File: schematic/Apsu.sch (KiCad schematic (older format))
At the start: 34 parts

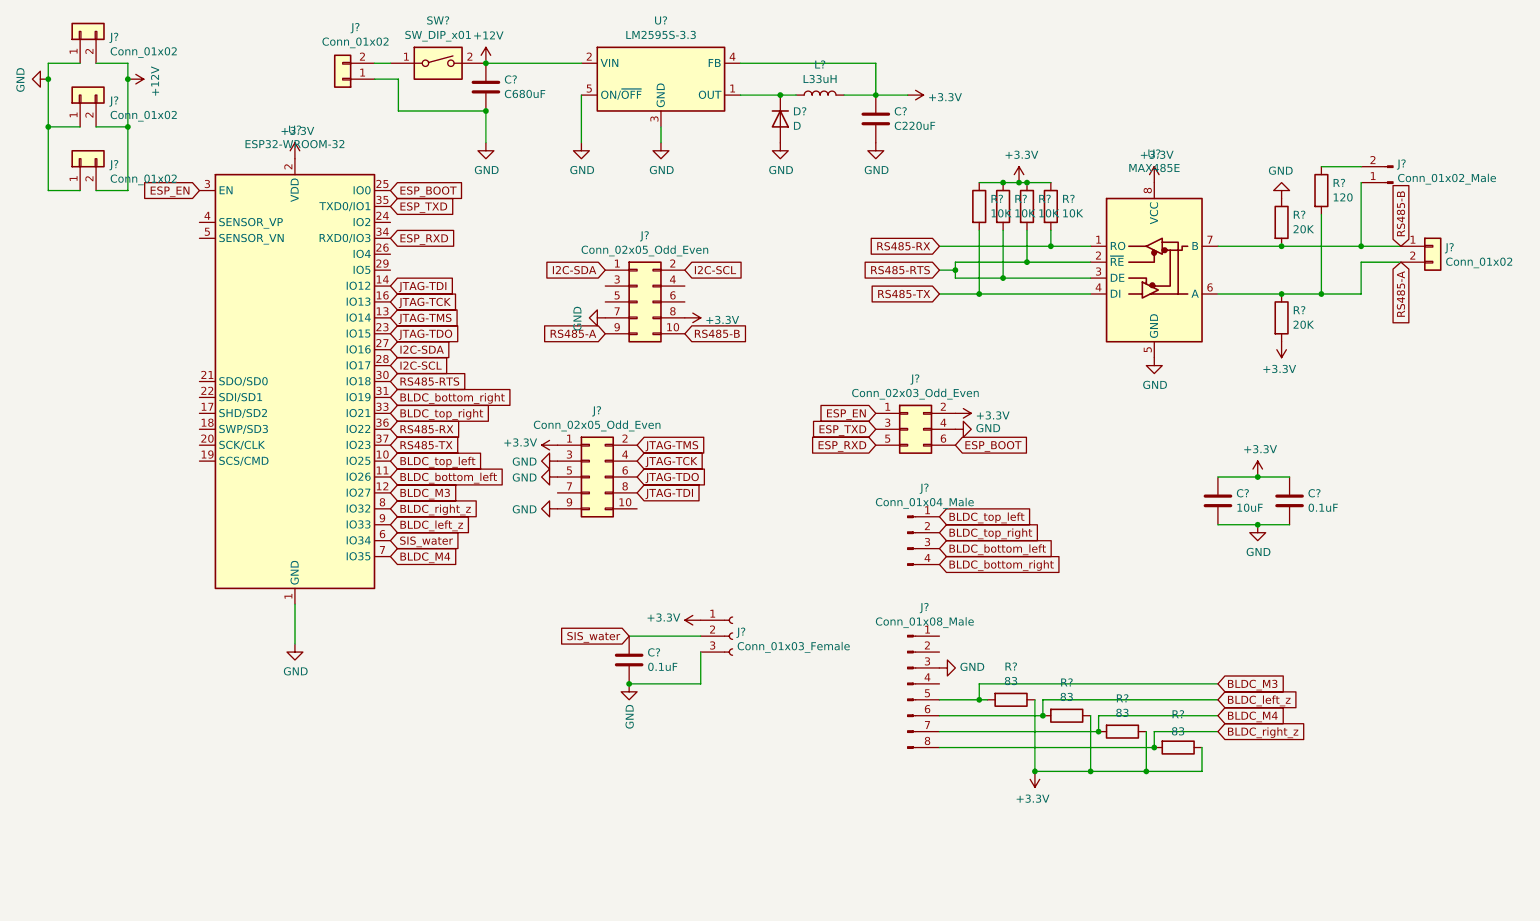
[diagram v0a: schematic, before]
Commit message: dingentjes
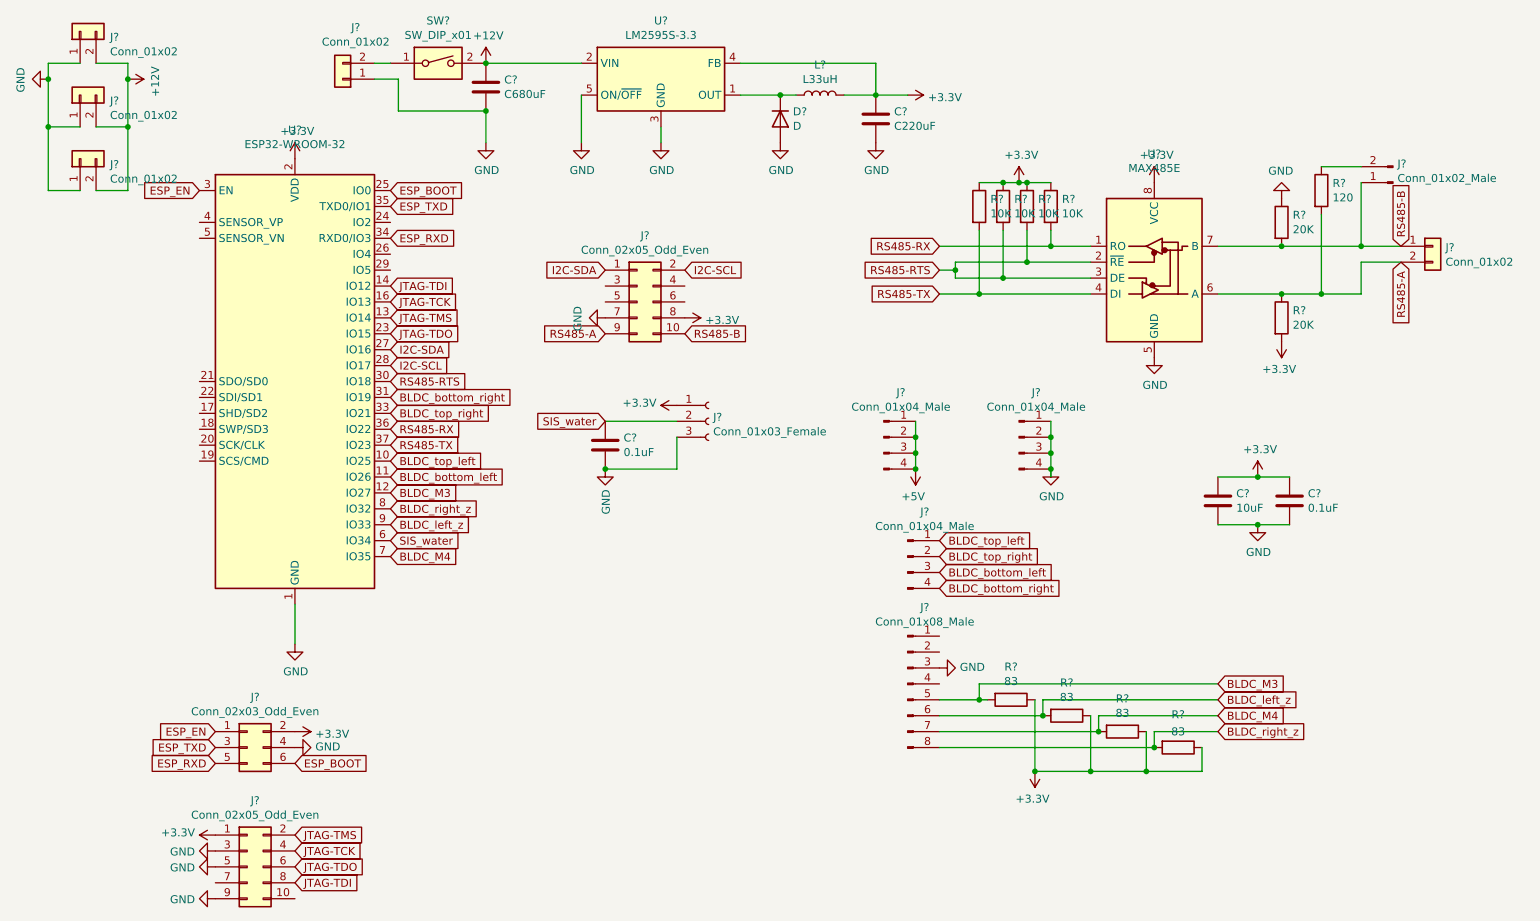
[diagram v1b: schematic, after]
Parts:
- added J? (x2): Conn_01x04_Male, symbol Connector:Conn_01x04_Male
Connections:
- net GND: now also J?.1 (Pin_1), J?.2 (Pin_2), J?.3 (Pin_3), J?.4 (Pin_4)
- new net +5V: J?.1 (Pin_1), J?.2 (Pin_2), J?.3 (Pin_3), J?.4 (Pin_4)
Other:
- moved on the sheet: C?, J?
